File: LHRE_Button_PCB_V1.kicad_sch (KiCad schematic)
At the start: 12 parts, among them J1 Conn_01x08_Male, SW1 SW_Push, SW2 SW_Push, SW3 SW_Push, SW4 SW_Push, SW5 SW_Push, SW6 SW_Push

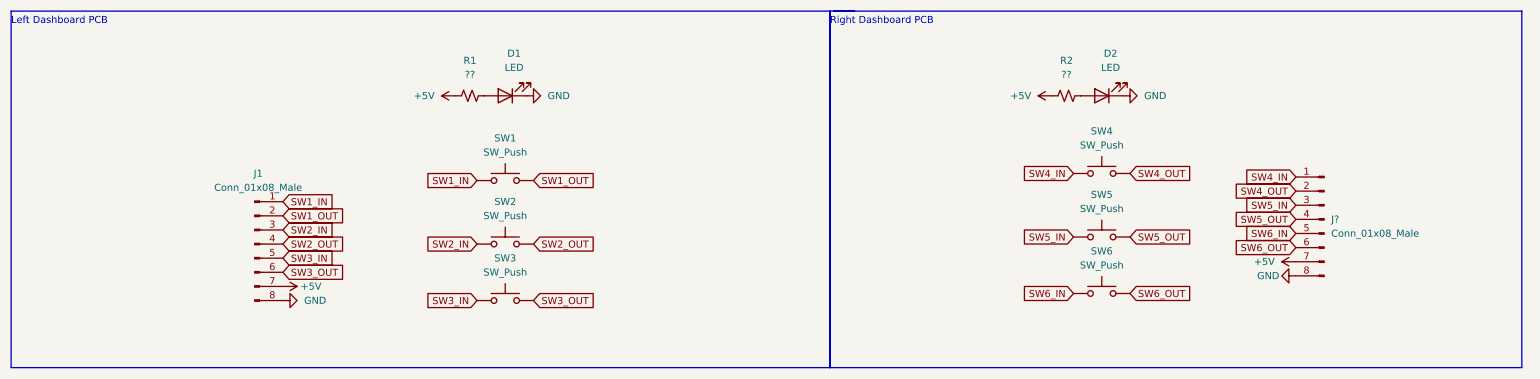
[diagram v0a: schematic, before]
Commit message: second review dash
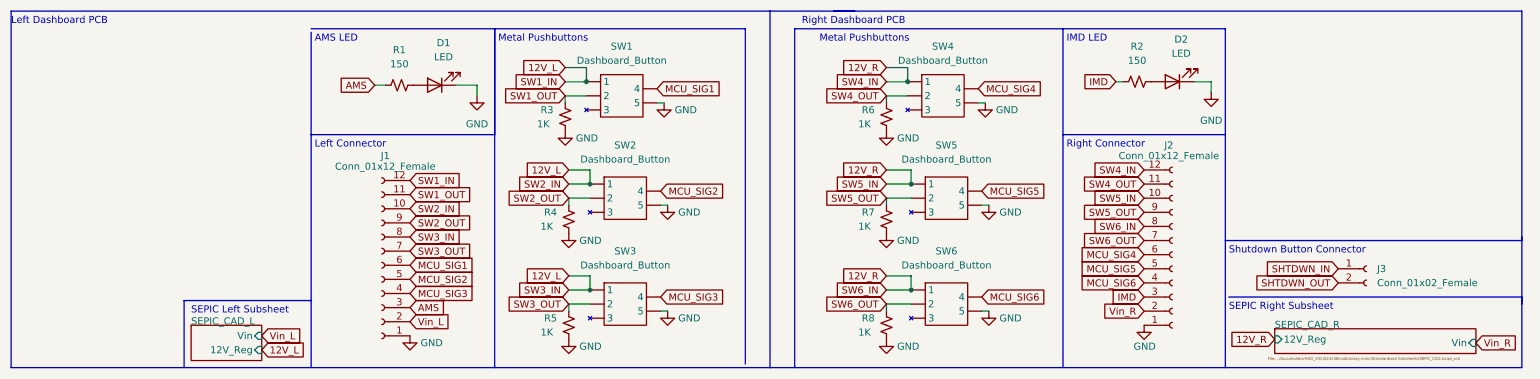
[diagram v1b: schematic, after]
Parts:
- removed J1, J?: Conn_01x08_Male, symbol Connector:Conn_01x08_Male
- removed SW1, SW2, SW3, SW4, SW5, SW6: SW_Push, symbol Switch:SW_Push
- added J1, J2: Conn_01x12_Female, symbol Connector:Conn_01x12_Female
- added J3: Conn_01x02_Female, symbol Connector:Conn_01x02_Female
- added R3, R4, R5, R6, R7, R8: 1K, Resistor_SMD:R_0201_0603Metric, symbol Device:R_Small_US
- added SW1, SW2, SW3, SW4, SW5, SW6: Dashboard_Button, Dashboard_LED:Dashboard_Btn, symbol Dashboard:Dashboard_Button
- D1, D2: footprint (none) -> Dashboard_LED:LEDC1608X80N
- R1, R2: value ?? -> 150; footprint (none) -> Resistor_SMD:R_0201_0603Metric
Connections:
- net GND: now also J1.1 (Pin_1), J2.1 (Pin_1), R3.1, R4.1, R5.1, R6.1, R7.1, R8.1, SW1. (5), SW2. (5), SW3. (5), SW4. (5), SW5. (5), SW6. (5)
- net SW1_OUT: now also J1.11 (Pin_11), R3.2, SW1. (5)
- net SW2_OUT: now also J1.9 (Pin_9), R4.2, SW2. (5)
- net SW3_OUT: now also J1.7 (Pin_7), R5.2, SW3. (5)
- net SW4_OUT: now also J2.11 (Pin_11), R6.2, SW4. (5)
- net SW5_OUT: now also J2.9 (Pin_9), R7.2, SW5. (5)
- net SW6_OUT: now also J2.7 (Pin_7), R8.2, SW6. (5)
- net +5V renamed AMS
- net AMS: now also J1.3 (Pin_3); no longer R2.1
- new net 12V_L: J1.10 (Pin_10), J1.12 (Pin_12), J1.8 (Pin_8), SW1. (5), SW2. (5), SW3. (5)
- new net 12V_R: J2.10 (Pin_10), J2.12 (Pin_12), J2.8 (Pin_8), SW4. (5), SW5. (5), SW6. (5)
- new net IMD: J2.3 (Pin_3), R2.1
- new net MCU_SIG1: J1.6 (Pin_6), SW1. (5)
- new net MCU_SIG2: J1.5 (Pin_5), SW2. (5)
- new net MCU_SIG3: J1.4 (Pin_4), SW3. (5)
- new net MCU_SIG4: J2.6 (Pin_6), SW4. (5)
- new net MCU_SIG5: J2.5 (Pin_5), SW5. (5)
- new net MCU_SIG6: J2.4 (Pin_4), SW6. (5)
- new net SHTDWN_IN: J3.1 (Pin_1)
- new net SHTDWN_OUT: J3.2 (Pin_2)
- new net Vin_L: J1.2 (Pin_2)
- new net Vin_R: J2.2 (Pin_2)
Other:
- added sheet SEPIC_CAD_L (../AccumulatorHUD_2023/2023KicadLibrary-main/Standardized Subsheets/SEPIC_CAD.kicad_sch)
- added sheet SEPIC_CAD_R (../AccumulatorHUD_2023/2023KicadLibrary-main/Standardized Subsheets/SEPIC_CAD.kicad_sch)
- note added: "AMS LED"
- note added: "IMD LED"
- note added: "Left Connector"
- note added: "Metal Pushbuttons"
- note added: "Right Connector"
- note added: "SEPIC Left Subsheet"
- note added: "SEPIC Right Subsheet"
- note added: "Shutdown Button Connector"
- moved on the sheet: D1, D2, R1, R2
